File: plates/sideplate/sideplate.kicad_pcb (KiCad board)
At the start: 2 copper layers, 107.2 x 33.2 mm, 2 parts

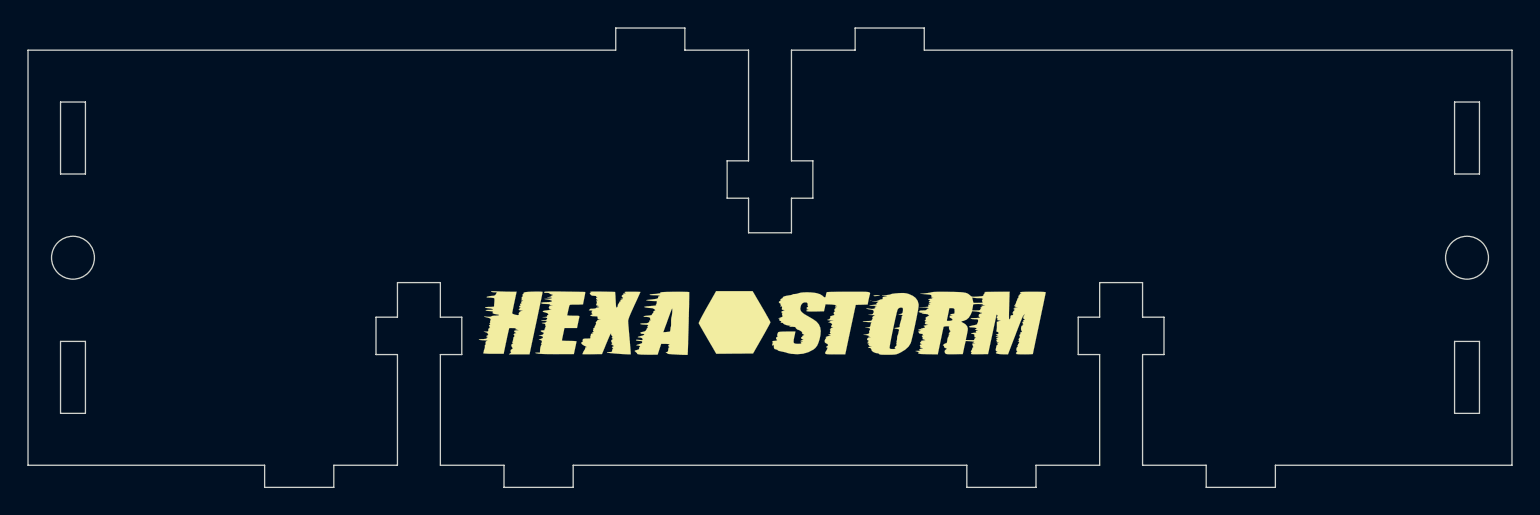
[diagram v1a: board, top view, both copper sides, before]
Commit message: added design of june
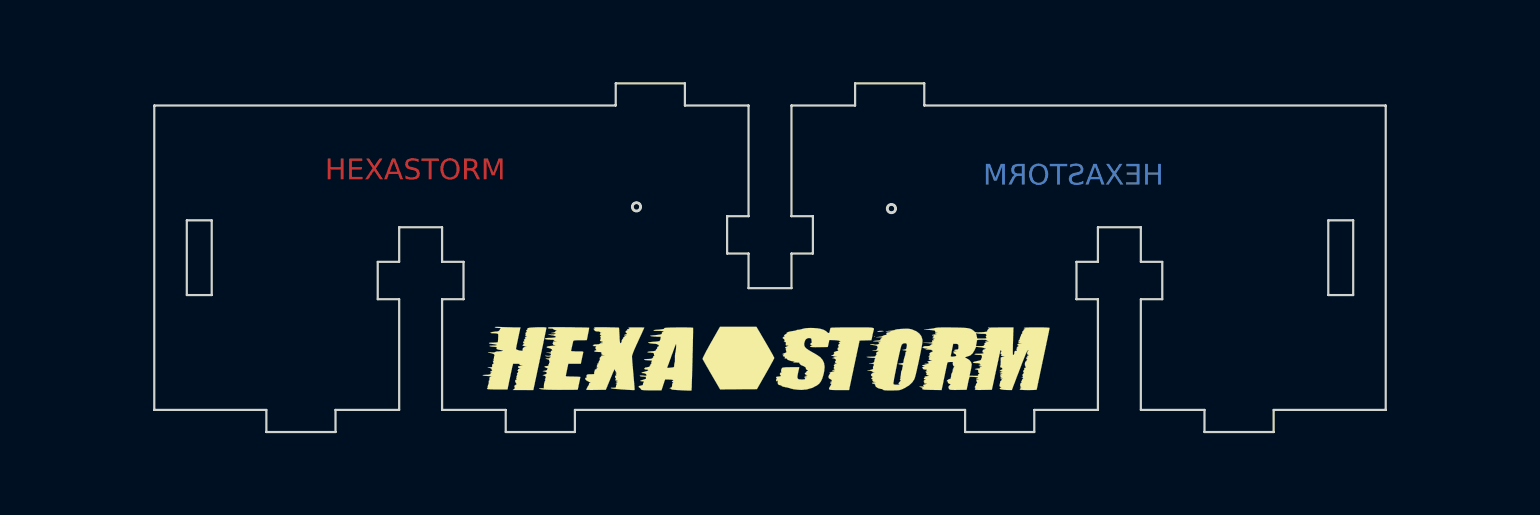
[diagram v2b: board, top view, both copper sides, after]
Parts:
- moved L1 2.59 mm to (153.8, 111.2)
- moved L2 2.59 mm to (154.4, 111.2)
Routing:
- net (no net): vias 0 -> 2
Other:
- board size 107.2 x 33.2 mm -> 89 x 25.2 mm
- net class Default removed
- board text added: "HEXASTORM"
